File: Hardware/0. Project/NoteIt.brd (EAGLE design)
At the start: 50 x 35 mm, 61 parts, among them CN1 USB 3.2 Gen 2 Type C Receptac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, CN3 Micro-SD Card, CN4 FTSH-105-01-L-DV-K-TR, CN6 Lithium Ion Polymer, IC5 S-8261ACMMD-G4MT2U, P1 OSTTE020104, Q1 SI2374DS, Q2 SI2374DS, SW1 KY-040, U1 SN74AHC1G125DBV, U2 GL823K, U3 TLV75530PDBVR, U4 TS3A27518EPWR, U8 DS3231/SO

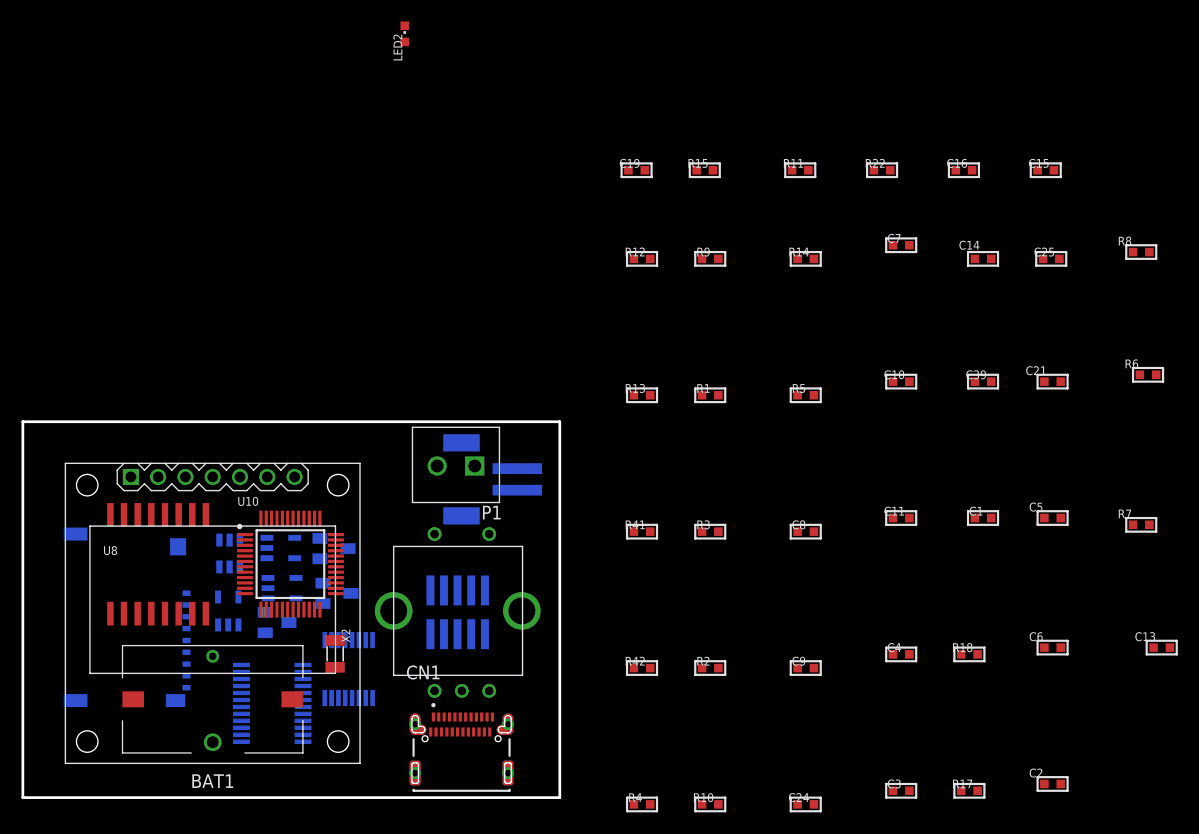
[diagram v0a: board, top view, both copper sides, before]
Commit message: Board design WIP
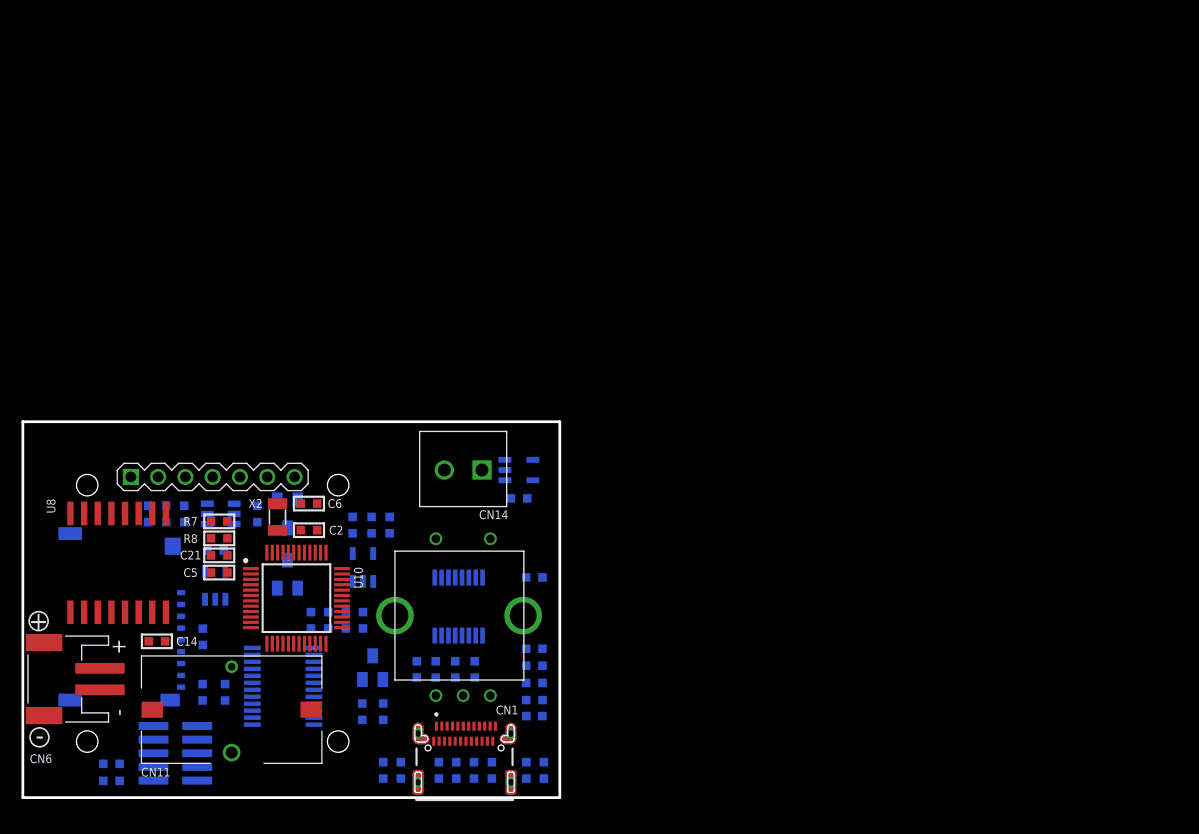
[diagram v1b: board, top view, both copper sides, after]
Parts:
- removed BAT1: CR1220, SamacSys_Parts:1072
- removed P1: OSTTE020104, Terminal Block 2P 3.5pitch:OST_OSTTE020104
- added C12: (no value), My-RLC:C0603
- added CN11: CR1220, SamacSys_Parts:1072
- added CN14: OSTTE020104, Terminal Block 2P 3.5pitch:OST_OSTTE020104
- added R16, R19, R20: (no value), My-RLC:R0603
- moved R6 103.7 mm to (8.26, 1.56), flipped to the bottom
- moved C13 98.4 mm to (8.26, 3.15), flipped to the bottom, turned to 180 degrees
- moved R8 89.9 mm to (18.3, 24.1)
- moved C25 87.4 mm to (11.7, 26.4), flipped to the bottom, turned to 270 degrees
- moved R7 85.9 mm to (18.3, 25.7)
- moved C14 84.8 mm to (12.5, 14.6), turned to 180 degrees
- moved C21 79.3 mm to (18.3, 22.6), turned to 180 degrees
- moved C5 77.8 mm to (18.3, 21.0), turned to 180 degrees
- moved C16 76.6 mm to (35.2, 2.54), flipped to the bottom, turned to 90 degrees
- moved C2 73.2 mm to (26.6, 24.9)
- moved R22 72.4 mm to (15.0, 26.4), flipped to the bottom, turned to 270 degrees
- moved C6 70.5 mm to (26.6, 27.4)
- moved C7 68.7 mm to (33.6, 2.54), flipped to the bottom, turned to 90 degrees
- moved C3 66.6 mm to (16.8, 15.0), flipped to the bottom, turned to 90 degrees
- moved LED2 64.7 mm to (47.6, 7.59), flipped to the bottom, turned to 270 degrees
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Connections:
- net 0V: now also C12.2, CN11.-, CN14.2; no longer BAT1.-, P1.2
- net 3.3V: now also C12.1, R16.1, R19.1, R20.1
- net GPIO_ROTARY_ENCODER_BUTTON: now also R16.2
- net GPIO_ROTARY_ENCODER_SIGNAL_A: now also R19.2
- net GPIO_ROTARY_ENCODER_SIGNAL_B: now also R20.2
- net N$22: now also CN11.+; no longer BAT1.+
- net N$4: now also CN14.1; no longer P1.1
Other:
- board text added: "+"
- board text added: "-"
